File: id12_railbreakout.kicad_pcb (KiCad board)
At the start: 2 copper layers, 84.1 x 26.7 mm, 16 parts, among them J1 RJ45, P1 CONN_4, U1 LM1117, U2 ID-12

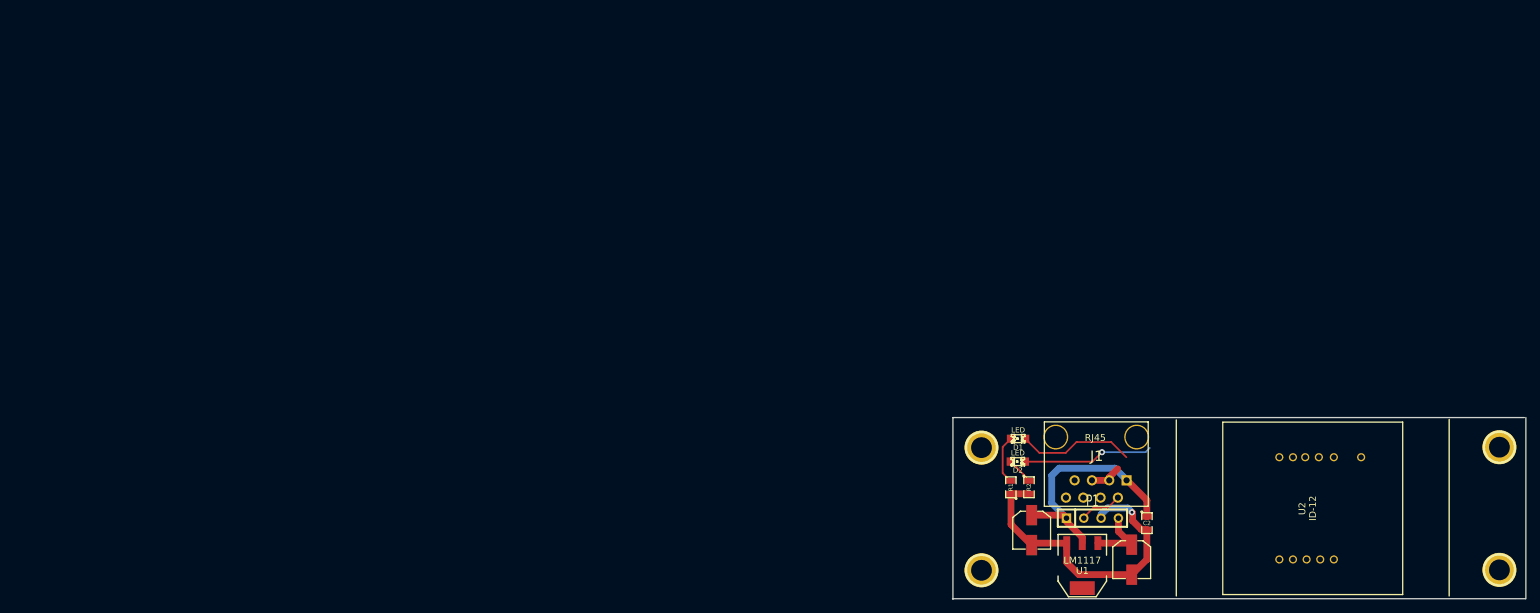
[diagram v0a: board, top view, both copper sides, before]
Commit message: Small fixes and board layout
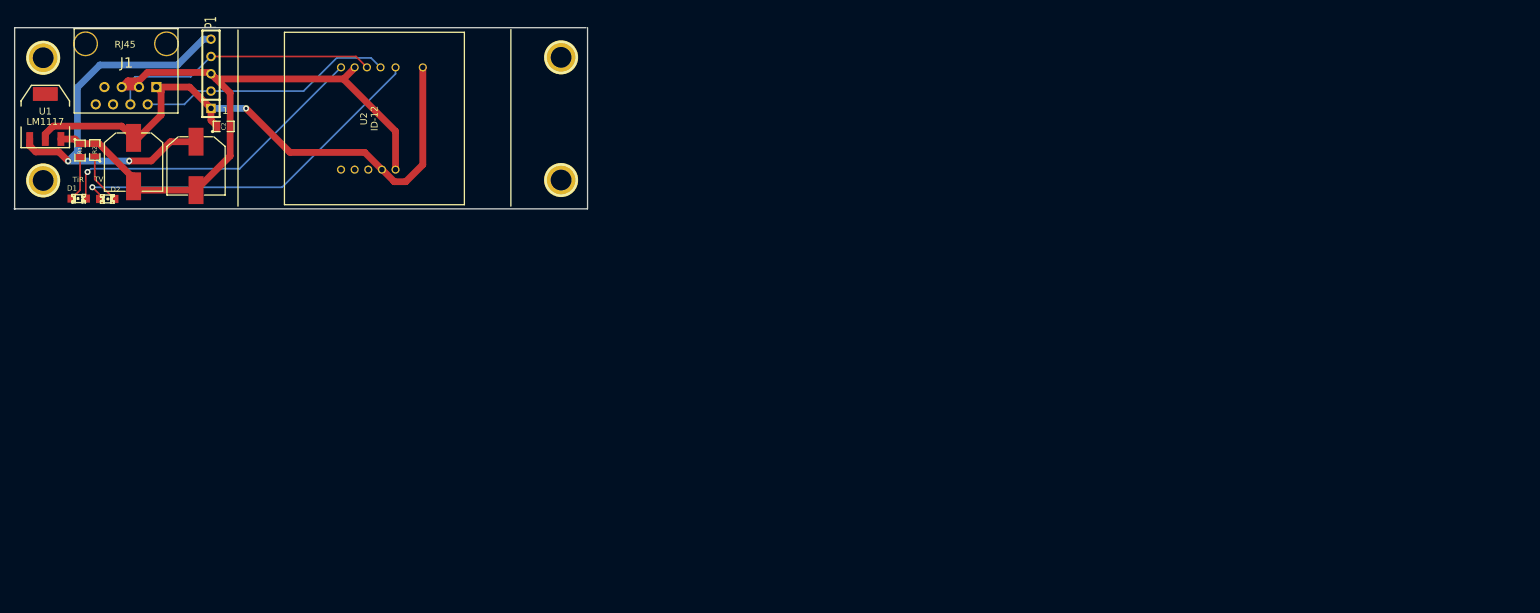
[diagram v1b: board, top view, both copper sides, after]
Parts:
- C1, C3: footprint c-smd-5mmx6.1mm -> c-smd-8mmx10.5mm
- D1: value LED -> TiR
- D2: value LED -> TV
- P1: value CONN_4 -> CONN_5; footprint SIL-4 -> SIL-5
- moved U1 165.8 mm to (86.6, 97.4), turned to 0 degrees
- moved J1 153.6 mm to (98.5, 86.8)
- moved ? 149.9 mm to (105.6, 109.8)
- moved ? 149.1 mm to (86.3, 88.8)
- moved ? 149.1 mm to (86.3, 106.8)
- moved ? 149.1 mm to (162.3, 106.7)
- moved ? 149.1 mm to (162.3, 88.7)
- moved U2 149.1 mm to (134.9, 97.7)
- moved C1 148.9 mm to (108.8, 104.7)
- moved C2 147.4 mm to (112.8, 98.9), turned to 0 degrees
- moved R2 145.7 mm to (93.9, 102.3), turned to 90 degrees
- moved P1 145.4 mm to (111.0, 89.9), turned to 90 degrees
- moved R1 145.2 mm to (91.7, 102.4), turned to 270 degrees
- moved C3 142.4 mm to (99.6, 104.1)
- moved D1 142.3 mm to (91.5, 109.5)
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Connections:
- J1 pad 4: (no net) -> N-000007
- P1 pad 4: VAA -> N-000007
- U2 pad 9: (no net) -> N-000007
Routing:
- net VAA: track 9.10 -> 61.4 mm, vias 0 -> 2
- net VCC: track 35.9 -> 87.9 mm, vias 0 -> 1
- net VSS: track 51.5 -> 99.3 mm, vias 1 -> 0
- net N-000007: track 0.00 -> 40.2 mm
- net N-000008: track 19.2 -> 54.5 mm
- net N-000006: track 6.32 -> 37.6 mm
- net N-000003: track 17.3 -> 47.6 mm, vias 0 -> 1
- net N-000001: track 3.92 -> 7.42 mm
- net N-000002: track 7.21 -> 6.62 mm
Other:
- board text added: "1"
- board text added: "Board: Dirkjan Krijnders https://github.com/dirkjankrijnders/id12_trackbreakout"
- board text added: "P1: 1. Vcc 2. D1 3. GND 4. D0 5. PWR"
- board text removed: "Board: Dirkjan Krijnders http://github.com"
